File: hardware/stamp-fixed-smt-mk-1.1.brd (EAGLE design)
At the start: 22.9 x 17.8 mm, 13 parts, among them U1_ ROTARY_ENCODER_SWITCH, U2 Tiny85

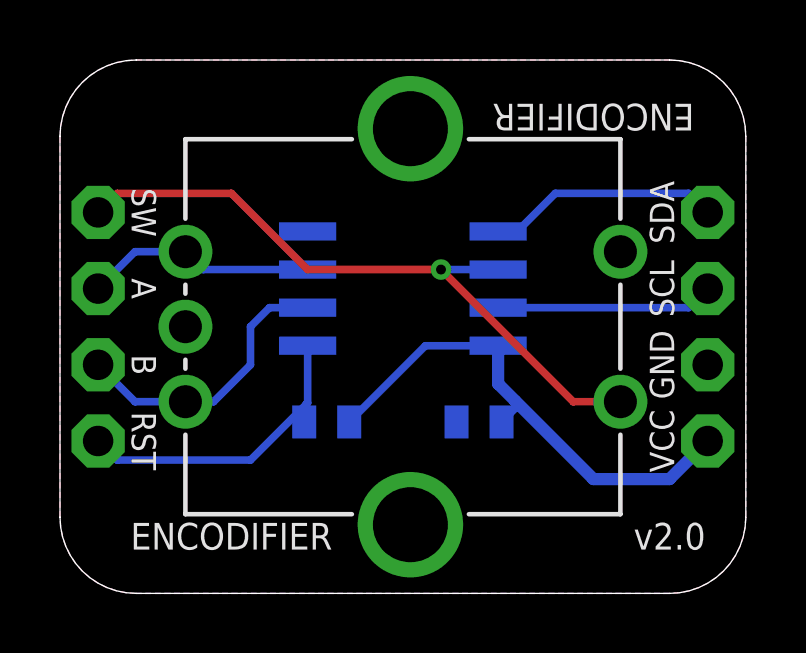
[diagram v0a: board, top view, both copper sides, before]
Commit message: have some boards, dawg
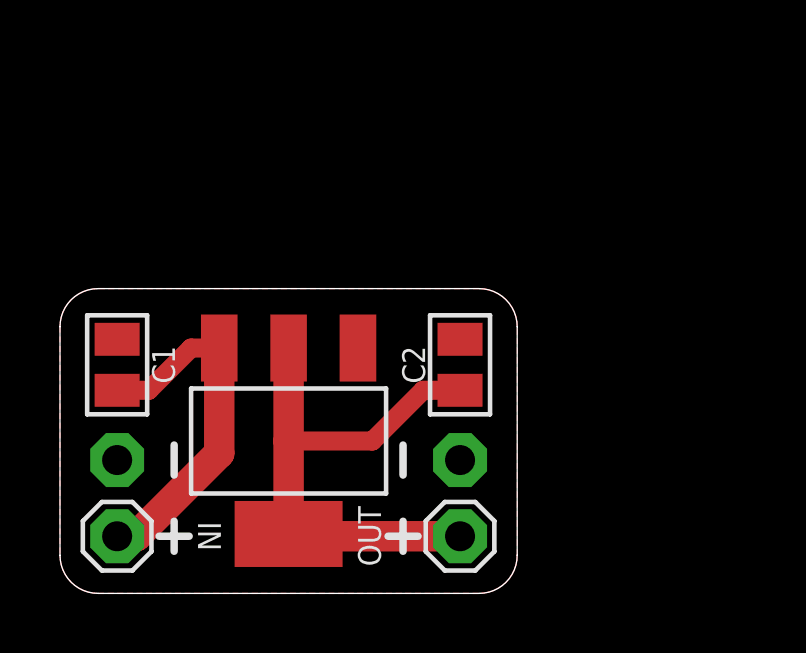
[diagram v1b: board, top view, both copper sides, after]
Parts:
- removed A, B, GND, RST, SCL, SDA, SW, VCC: M01PTH-1MM, a_parts:1X01-1MM-NS
- removed R1: 10k, a_parts:R0603-TIGHTER
- removed U1_: ROTARY_ENCODER_SWITCH, a_parts:ROTARY_ENCODER_SWITCH
- removed U2: Tiny85, a_parts:SO08-EIAJ
- added C2: 22u, a_parts:C0805-TIGHTER
- added IN: M02PTH-CENTERED-L+, a_parts:1X02-CENTER-L+
- added OUT: M02PTH-CENTERED-R+, a_parts:1X02-CENTER-R+
- added U1: LD1117, a_parts:SOT223
- C1: value 100n -> 4u7; device a_parts:C0603-TIGHTER -> a_parts:C0805-TIGHTER
- FRAME1: device A_butts:DUMMY -> a_parts:DUMMY
- moved C1 12.2 mm to (1.91, 7.62), flipped to the top, turned to 90 degrees
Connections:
- removed net A: A.1, U1_.A, U2.3
- removed net B: B.1, U1_.B, U2.2
- removed net MOSI/SDA: SDA.1, U2.5
- removed net RST: R1.1, RST.1, U2.1
- removed net SCK/SCL: SCL.1, U2.7
- removed net SW: SW.1, U1_.SW1, U2.6
- removed net VCC: C1.1, R1.2, U2.8, VCC.1
- new net VIN: C1.1, IN.1, U1.3
- new net VOUT: C2.1, OUT.2, U1.2, U1.4
- net GND: now also C2.2, IN.2, OUT.1, U1.1; no longer GND.1, U1_.C, U1_.SW2, U2.4
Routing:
- net SW: track 22.5 -> 0.00 mm, vias 1 -> 0
- net VOUT: track 0.00 -> 18.4 mm
- net VCC: track 17.0 -> 0.00 mm
- net VIN: track 0.00 -> 12.0 mm
- net RST: track 10.5 -> 0.00 mm
- net B: track 9.54 -> 0.00 mm
- net MOSI/SDA: track 7.77 -> 0.00 mm
- net A: track 7.74 -> 0.00 mm
- net SCK/SCL: track 7.25 -> 0.00 mm
- removed copper zone on layer 16, net GND
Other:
- board size 22.9 x 17.8 mm -> 15.2 x 10.2 mm
- board text added: "Postage Stamp V Reg"
- board text removed: "A"
- board text removed: "B"
- board text removed: "C"
- board text removed: "COM"
- board text removed: "ENCODIFIER"
- board text removed: "SW"
